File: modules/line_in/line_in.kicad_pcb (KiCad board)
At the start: 2 copper layers, 27.9 x 66 mm, 24 parts, among them U1 LM358, U2 LM358, U3 LM358

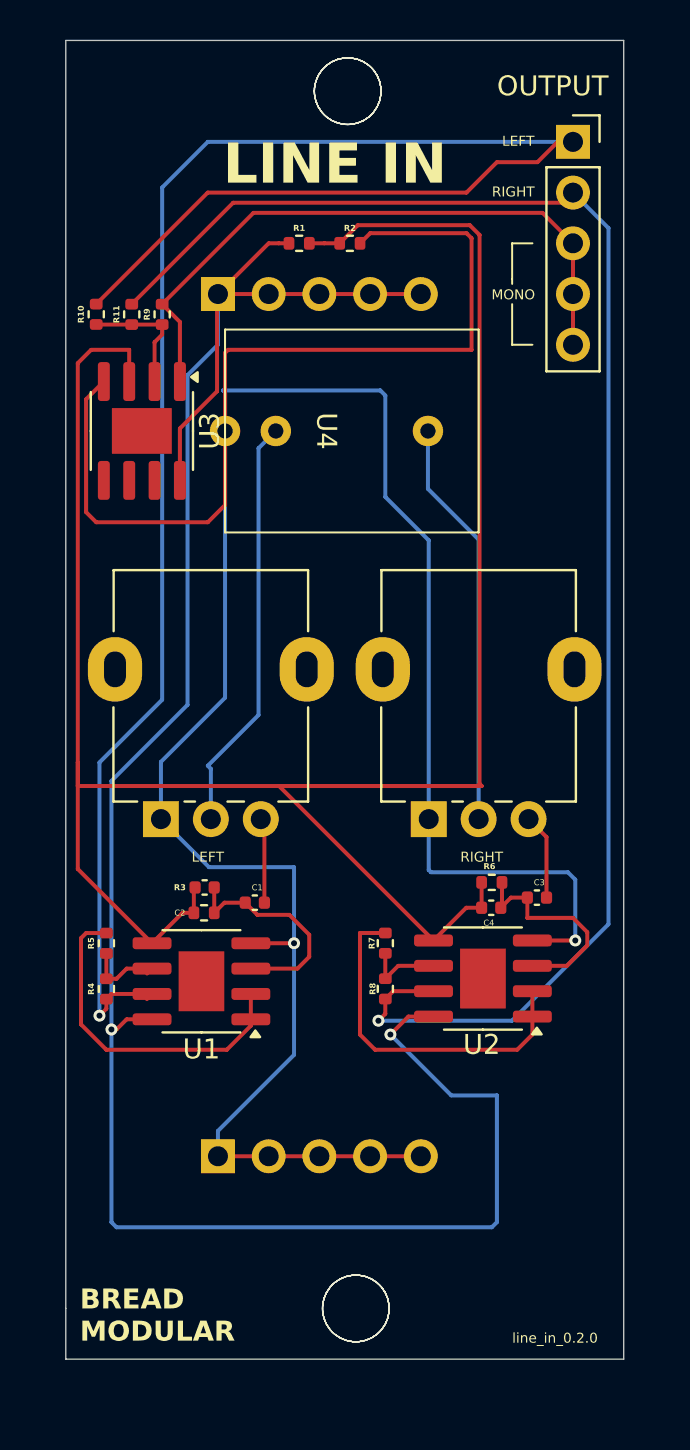
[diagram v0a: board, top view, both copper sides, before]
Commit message: Start working on the new version of line_in
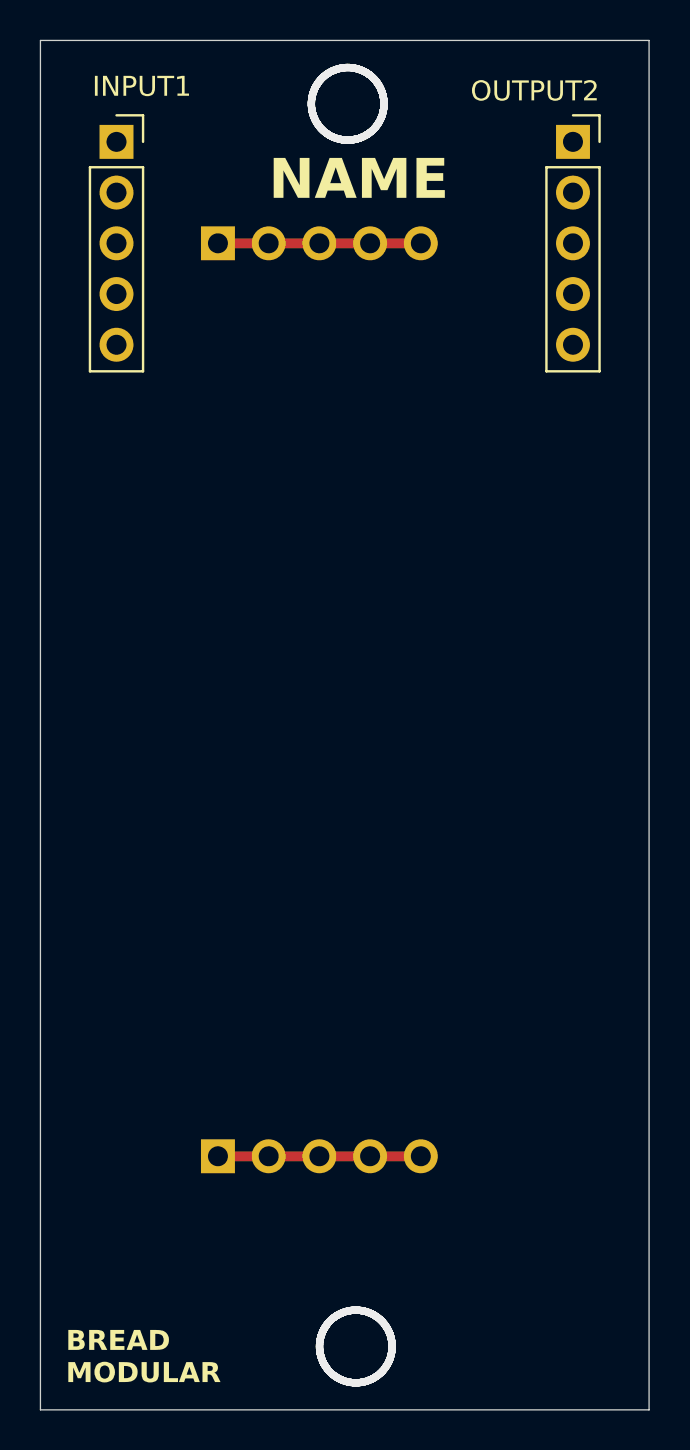
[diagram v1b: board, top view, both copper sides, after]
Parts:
- removed C1, C3: 0.1uf, Capacitor_SMD:C_0402_1005Metric
- removed C2, C4: 33pf, Capacitor_SMD:C_0402_1005Metric
- removed LEFT, RIGHT: 100K, Potentiometer_THT:Potentiometer_Alpha_RD901F-40-00D_Single_Vertical
- removed OUTPUT: Outputs, Connector_PinSocket_2.54mm:PinSocket_1x05_P2.54mm_Vertical
- removed R1, R2: 1K, Resistor_SMD:R_0402_1005Metric
- removed R10, R11, R3, R4, R6, R8: 100K, Resistor_SMD:R_0402_1005Metric
- removed R5, R7: 10K, Resistor_SMD:R_0402_1005Metric
- removed R9: 51K, Resistor_SMD:R_0402_1005Metric
- removed U1, U2, U3: LM358, Package_SO:SOIC-8-1EP_3.9x4.9mm_P1.27mm_EP2.29x3mm
- removed U4: ~, Footprints:Audio_Socket_TRS_3.5mm
- added INPUT1: Conn_01x05_Socket, Connector_PinSocket_2.54mm:PinSocket_1x05_P2.54mm_Vertical, F.Cu at (50.8, 45.7)
- added OUTPUT2: Conn_01x05_Socket, Connector_PinSocket_2.54mm:PinSocket_1x05_P2.54mm_Vertical, F.Cu at (73.7, 45.7)
- moved 5V1 2.54 mm to (55.9, 50.8)
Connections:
- net +5V renamed Net-(5V1-Pin_1)
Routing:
- net GND: track 150.5 -> 10.2 mm, vias 2 -> 0
- net 2.5V: track 112.5 -> 0.00 mm
- net Net-(5V1-Pin_1): track 110.8 -> 10.2 mm, vias 2 -> 0
- net OUT_L: track 95.3 -> 0.00 mm, vias 1 -> 0
- net OUT_R: track 79.1 -> 0.00 mm, vias 1 -> 0
- net OUT_MONO: track 32.4 -> 0.00 mm
- net Net-(U4-TIP): track 20.9 -> 0.00 mm
- net Net-(U4-RING): track 20.5 -> 0.00 mm
- net Net-(U2A--): track 17.8 -> 0.00 mm
- net Net-(U1A--): track 16.8 -> 0.00 mm
- net Net-(U1A-+): track 11.2 -> 0.00 mm
- net Net-(U2A-+): track 11.0 -> 0.00 mm
- net Net-(U3A--): track 6.32 -> 0.00 mm
- net IN R: track 4.30 -> 0.00 mm
- net IN L: track 4.26 -> 0.00 mm
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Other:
- board size 27.9 x 66 mm -> 30.5 x 68.6 mm
- board text added: "NAME"
- board text removed: "LEFT"
- board text removed: "LINE IN"
- board text removed: "MONO"
- board text removed: "RIGHT"
- board text removed: "line_in_0.2.0"
